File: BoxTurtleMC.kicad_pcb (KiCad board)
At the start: 2 copper layers, 110 x 60 mm, 35 parts, among them M1 Conn_01x02 Pin1+ Pin2-, M2 Conn_01x02 Pin1+ Pin2-, M3 Conn_01x02 Pin1+ Pin2-, M4 Conn_01x02 Pin1+ Pin2-, M5 Conn_01x02 Pin1+ Pin2-, M6 Conn_01x02 Pin1+ Pin2-, M7 Conn_01x02 Pin1+ Pin2-, M8 Conn_01x02 Pin1+ Pin2-, SW1 Conn_01x02 Pin1+ Pin2-, SW2 Conn_01x02 Pin1+ Pin2-, SW3 Conn_01x02 Pin1+ Pin2-, SW4 Conn_01x02 Pin1+ Pin2-, SW5 Conn_01x02 Pin1+ Pin2-, SW6 Conn_01x02 Pin1+ Pin2-, U1 CJMCU-1051_TJA1051_CAN_Transc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, U2 Pico

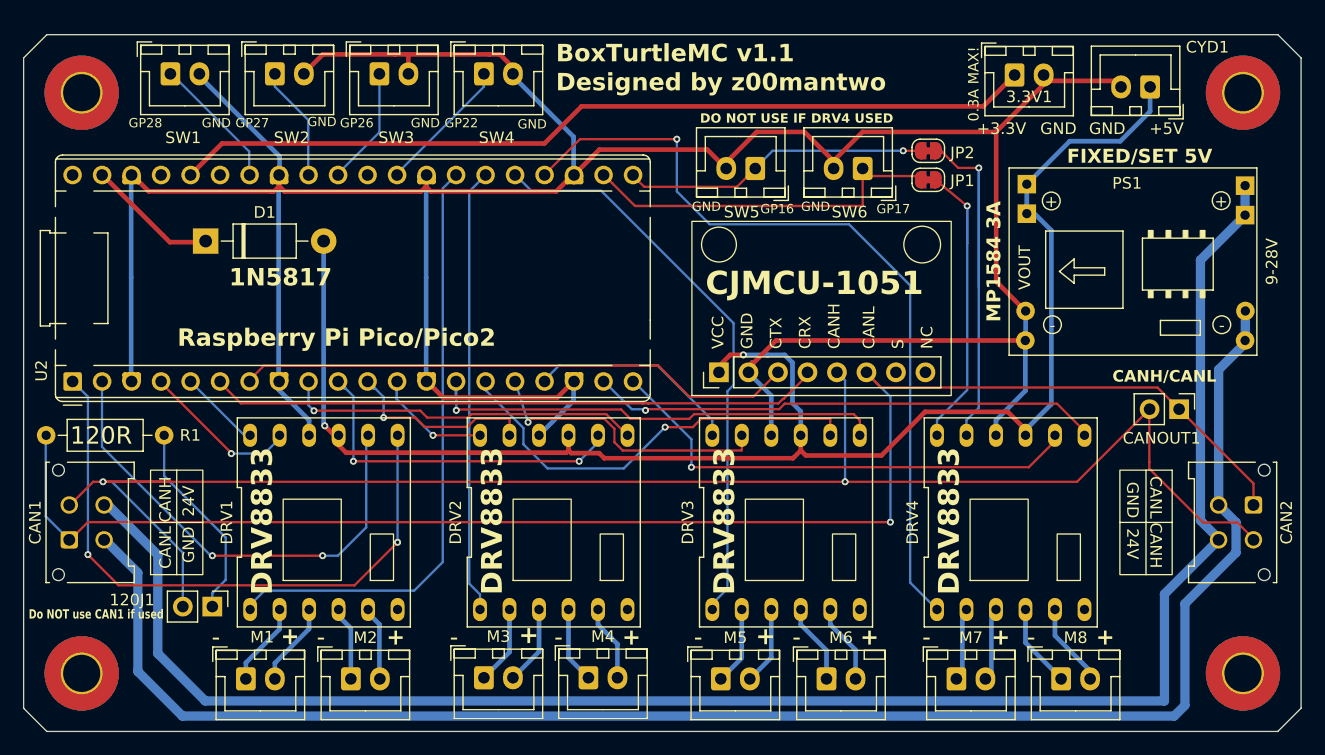
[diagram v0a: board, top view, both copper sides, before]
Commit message: Add files via upload
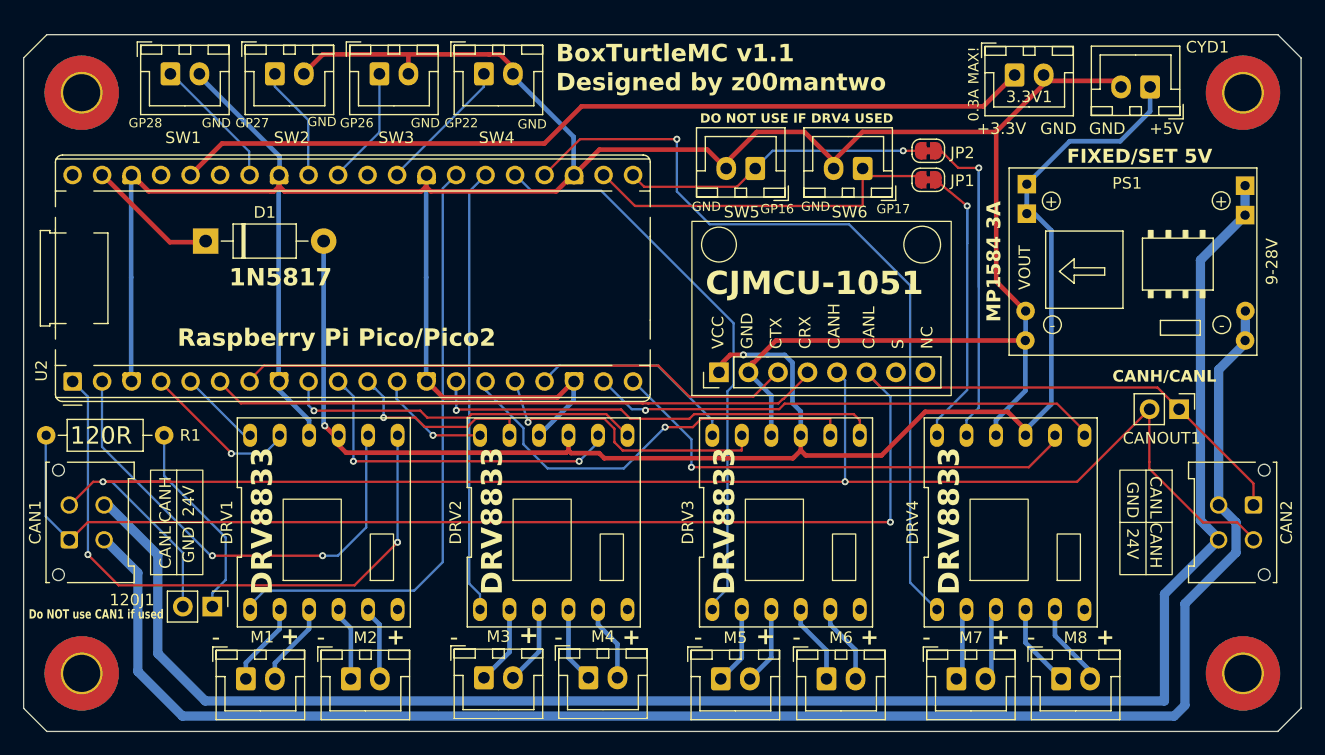
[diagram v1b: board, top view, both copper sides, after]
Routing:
- net GND: track 262.5 -> 259.4 mm
- net Net-(DRV1-AIN1): track 54.9 -> 54.0 mm
- net Net-(U1-CRX): track 53.3 -> 52.4 mm
- net Net-(DRV2-BOUT2): track 7.47 -> 6.57 mm
- net Net-(SW3-Pin_1): track 11.0 -> 10.2 mm
- net Net-(DRV3-BOUT1): track 7.67 -> 6.89 mm
